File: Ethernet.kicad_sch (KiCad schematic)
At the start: 2 parts, among them T1 WE-RJ45_7499010211A, U4 DP83825IRMQR

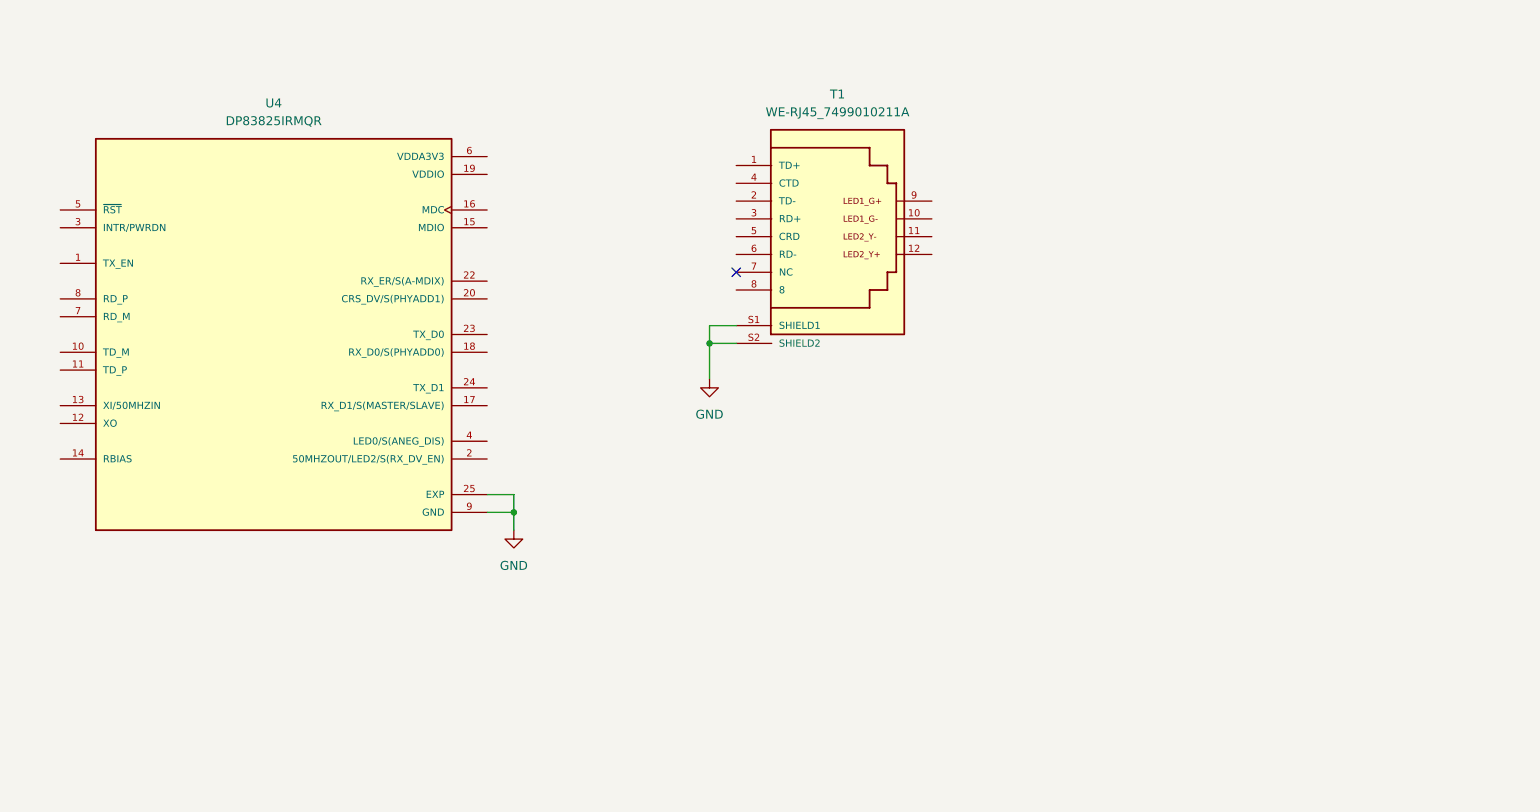
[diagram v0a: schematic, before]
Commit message: new
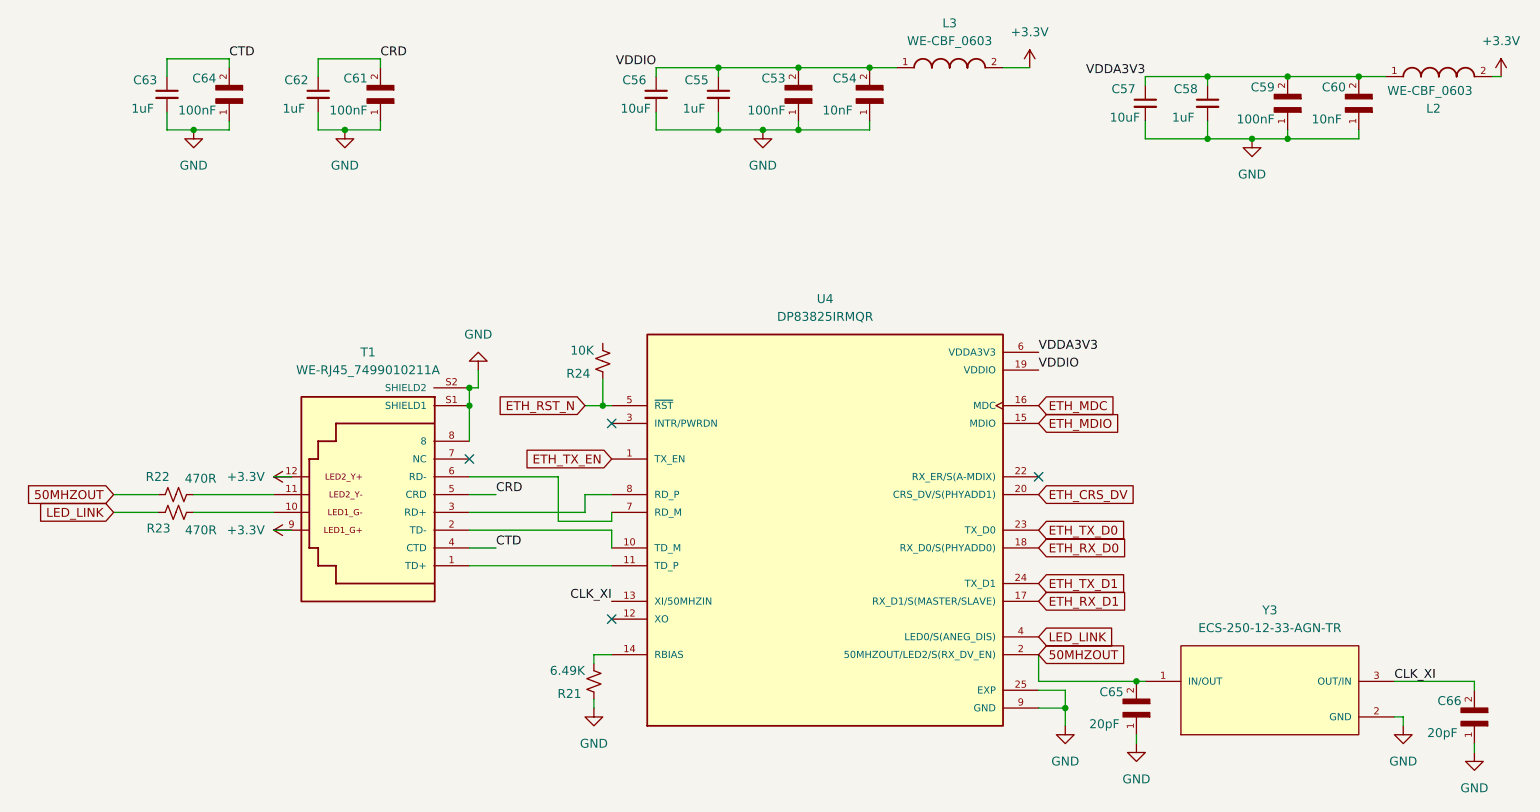
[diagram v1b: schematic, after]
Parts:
- added C53, C59, C61, C64: 100nF, C0402C104K4RAC:CAPC1005X55N, symbol C0402C104K4RAC:C0402C104K4RAC
- added C54, C60: 10nF, C0402C104K4RAC:CAPC1005X55N, symbol C0402C104K4RAC:C0402C104K4RAC
- added C55, C58, C62, C63: 1uF, Capacitor_SMD:C_0805_2012Metric, symbol Device:C_Small
- added C56, C57: 10uF, Capacitor_SMD:C_0805_2012Metric, symbol Device:C_Small
- added C65, C66: 20pF, C0402C104K4RAC:CAPC1005X55N, symbol C0402C104K4RAC:C0402C104K4RAC
- added L2, L3: WE-CBF_0603, GNSS_Library:WE-CBF_0603_W2.6, symbol WE-CBF_0603:WE-CBF_0603
- added R21: 6.49K, symbol Device:R_Small_US
- added R22, R23: 470R, symbol Device:R_Small_US
- added R24: 10K, symbol Device:R_Small_US
- added Y3: ECS-250-12-33-AGN-TR, GNSS_Library:XTAL_ECS-250-12-33-AGN-TR, symbol ECS-250-12-33-AGN-TR:ECS-250-12-33-AGN-TR
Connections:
- net EXP: now also T1.8, C53.1, C54.1, C55.2, C56.2, C57.2, C58.2, C59.1, C60.1, C61.1, C62.2, C63.2, C64.1, C65.1, C66.1, R21.1, Y3.2 (GND), Y3.4 (GND)
- net ETH_TX_EN: now reaches U4.1 (TX_EN)
- net at U4.10 (TD_M): now also T1.2 (TD-)
- net at U4.11 (TD_P): now also T1.1 (TD+)
- net CLK_XI: now reaches U4.13 (XI/50MHZIN)
- net CLK_XI: now also C66.2, Y3.3 (OUT/IN)
- net at U4.14 (RBIAS): now also R21.2
- net ETH_MDIO: now reaches U4.15 (MDIO)
- net ETH_MDC: now reaches U4.16 (MDC)
- net ETH_RX_D1: now reaches U4.17 (RX_D1/S(MASTER/SLAVE))
- net ETH_RX_D0: now reaches U4.18 (RX_D0/S(PHYADD0))
- net VDDIO: now reaches U4.19 (VDDIO)
- net VDDIO: now also C53.2, C54.2, C55.1, C56.1, L3.1
- net 50MHZOUT: now reaches U4.2 (50MHZOUT/LED2/S(RX_DV_EN))
- net 50MHZOUT: now also C65.2, R22.2, Y3.1 (IN/OUT)
- net ETH_CRS_DV: now reaches U4.20 (CRS_DV/S(PHYADD1))
- net ETH_TX_D0: now reaches U4.23 (TX_D0)
- net ETH_TX_D1: now reaches U4.24 (TX_D1)
- net LED_LINK: now reaches U4.4 (LED0/S(ANEG_DIS))
- net LED_LINK: now also R23.1
- net ETH_RST_N: now reaches U4.5 (~{RST})
- net ETH_RST_N: now also R24.1
- net VDDA3V3: now reaches U4.6 (VDDA3V3)
- net VDDA3V3: now also C57.1, C58.1, C59.2, C60.2, L2.1
- net at U4.7 (RD_M): now also T1.6 (RD-)
- net at U4.8 (RD_P): now also T1.3 (RD+)
- net at T1.10: now also R23.2
- net at T1.11: now also R22.1
- net +3.3V: now reaches T1.12
- net +3.3V: now also T1.9, L2.2, L3.2
- net CTD: now reaches T1.4 (CTD)
- net CTD: now also C63.1, C64.2
- net CRD: now reaches T1.5 (CRD)
- net CRD: now also C61.2, C62.1
- no-connect marks 1 -> 4
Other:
- moved on the sheet: T1, U4
